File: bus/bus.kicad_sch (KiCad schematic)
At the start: 3 parts, among them J1 Conn_01x02, J2 Conn_01x15, J3 Conn_01x08

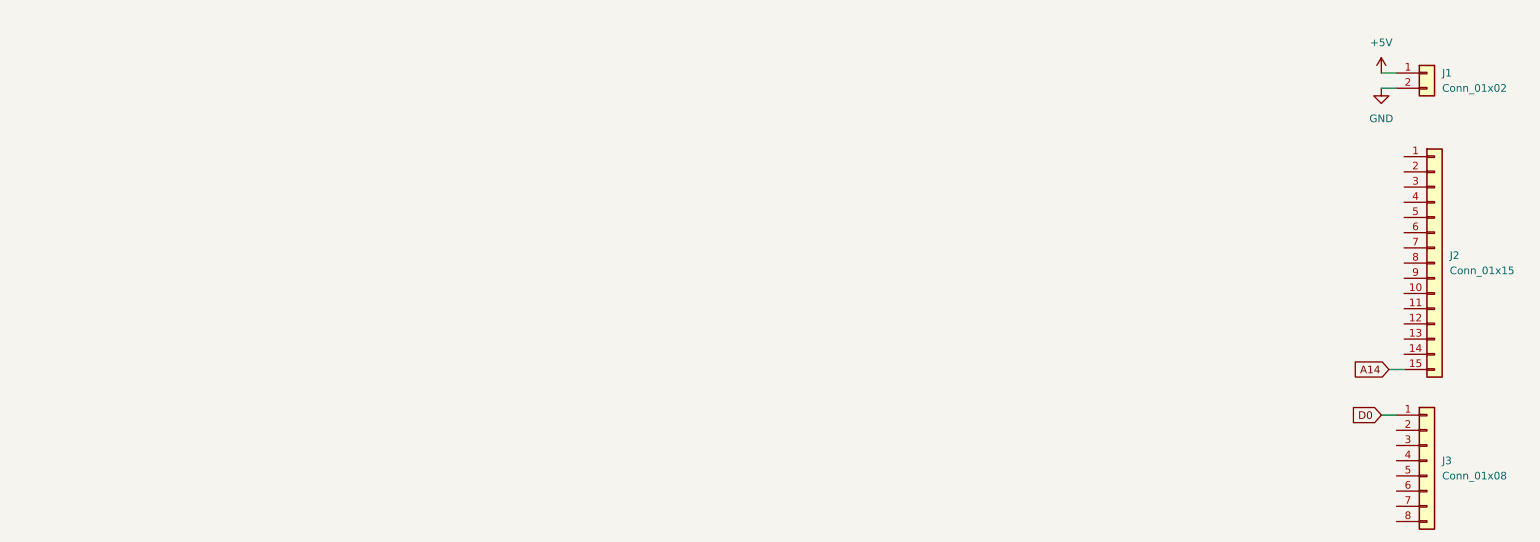
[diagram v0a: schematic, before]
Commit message: Done
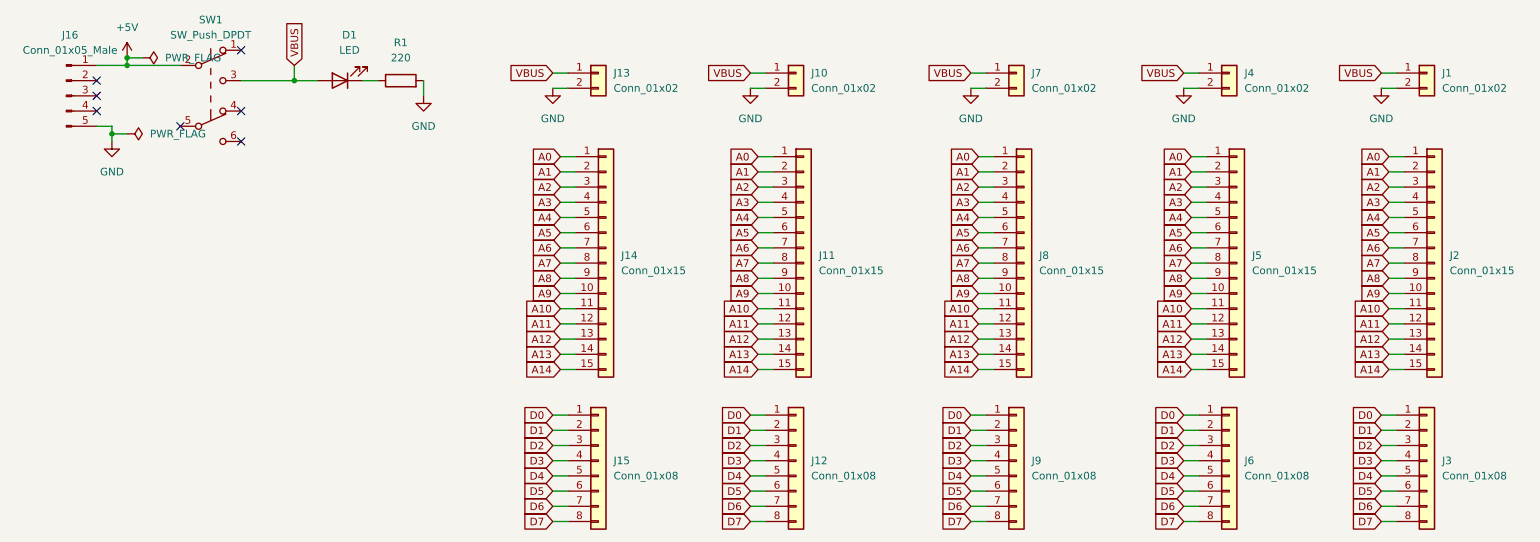
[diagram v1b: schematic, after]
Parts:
- added D1: LED, LED_THT:LED_D5.0mm, symbol Device:LED
- added J10, J13, J4, J7: Conn_01x02, Connector_PinSocket_2.54mm:PinSocket_1x02_P2.54mm_Vertical, symbol Connector_Generic:Conn_01x02
- added J11, J14, J5, J8: Conn_01x15, Connector_PinSocket_2.54mm:PinSocket_1x15_P2.54mm_Vertical, symbol Connector_Generic:Conn_01x15
- added J12, J15, J6, J9: Conn_01x08, Connector_PinSocket_2.54mm:PinSocket_1x08_P2.54mm_Vertical, symbol Connector_Generic:Conn_01x08
- added J16: Conn_01x05_Male, Connector_PinSocket_2.54mm:PinSocket_1x05_P2.54mm_Vertical, symbol Connector:Conn_01x05_Male
- added R1: 220, Resistor_THT:R_Axial_DIN0309_L9.0mm_D3.2mm_P12.70mm_Horizontal, symbol Device:R
- added SW1: SW_Push_DPDT, Button_Switch_THT:SW_E-Switch_EG1271_DPDT, symbol Switch:SW_Push_DPDT
- J1: footprint Connector_PinHeader_2.54mm:PinHeader_1x02_P2.54mm_Horizontal -> Connector_PinSocket_2.54mm:PinSocket_1x02_P2.54mm_Vertical
- J2: footprint Connector_PinHeader_2.54mm:PinHeader_1x15_P2.54mm_Horizontal -> Connector_PinSocket_2.54mm:PinSocket_1x15_P2.54mm_Vertical
- J3: footprint Connector_PinHeader_2.54mm:PinHeader_1x08_P2.54mm_Horizontal -> Connector_PinSocket_2.54mm:PinSocket_1x08_P2.54mm_Vertical
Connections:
- net +5V: now also J16.1 (Pin_1), SW1.2 (B); no longer J1.1 (Pin_1)
- net A14: now also J11.15 (Pin_15), J14.15 (Pin_15), J5.15 (Pin_15), J8.15 (Pin_15)
- net D0: now also J12.1 (Pin_1), J15.1 (Pin_1), J6.1 (Pin_1), J9.1 (Pin_1)
- net GND: now also J10.2 (Pin_2), J13.2 (Pin_2), J16.5 (Pin_5), J4.2 (Pin_2), J7.2 (Pin_2), R1.2
- net D1: now reaches J3.2 (Pin_2)
- net D1: now also J12.2 (Pin_2), J15.2 (Pin_2), J6.2 (Pin_2), J9.2 (Pin_2)
- net D2: now reaches J3.3 (Pin_3)
- net D2: now also J12.3 (Pin_3), J15.3 (Pin_3), J6.3 (Pin_3), J9.3 (Pin_3)
- net D3: now reaches J3.4 (Pin_4)
- net D3: now also J12.4 (Pin_4), J15.4 (Pin_4), J6.4 (Pin_4), J9.4 (Pin_4)
- net D4: now reaches J3.5 (Pin_5)
- net D4: now also J12.5 (Pin_5), J15.5 (Pin_5), J6.5 (Pin_5), J9.5 (Pin_5)
- net D5: now reaches J3.6 (Pin_6)
- net D5: now also J12.6 (Pin_6), J15.6 (Pin_6), J6.6 (Pin_6), J9.6 (Pin_6)
- net D6: now reaches J3.7 (Pin_7)
- net D6: now also J12.7 (Pin_7), J15.7 (Pin_7), J6.7 (Pin_7), J9.7 (Pin_7)
- net D7: now reaches J3.8 (Pin_8)
- net D7: now also J12.8 (Pin_8), J15.8 (Pin_8), J6.8 (Pin_8), J9.8 (Pin_8)
- net A0: now reaches J2.1 (Pin_1)
- net A0: now also J11.1 (Pin_1), J14.1 (Pin_1), J5.1 (Pin_1), J8.1 (Pin_1)
- net A9: now reaches J2.10 (Pin_10)
- net A9: now also J11.10 (Pin_10), J14.10 (Pin_10), J5.10 (Pin_10), J8.10 (Pin_10)
- net A10: now reaches J2.11 (Pin_11)
- net A10: now also J11.11 (Pin_11), J14.11 (Pin_11), J5.11 (Pin_11), J8.11 (Pin_11)
- net A11: now reaches J2.12 (Pin_12)
- net A11: now also J11.12 (Pin_12), J14.12 (Pin_12), J5.12 (Pin_12), J8.12 (Pin_12)
- net A12: now reaches J2.13 (Pin_13)
- net A12: now also J11.13 (Pin_13), J14.13 (Pin_13), J5.13 (Pin_13), J8.13 (Pin_13)
- net A13: now reaches J2.14 (Pin_14)
- net A13: now also J11.14 (Pin_14), J14.14 (Pin_14), J5.14 (Pin_14), J8.14 (Pin_14)
- net A1: now reaches J2.2 (Pin_2)
- net A1: now also J11.2 (Pin_2), J14.2 (Pin_2), J5.2 (Pin_2), J8.2 (Pin_2)
- net A2: now reaches J2.3 (Pin_3)
- net A2: now also J11.3 (Pin_3), J14.3 (Pin_3), J5.3 (Pin_3), J8.3 (Pin_3)
- net A3: now reaches J2.4 (Pin_4)
- net A3: now also J11.4 (Pin_4), J14.4 (Pin_4), J5.4 (Pin_4), J8.4 (Pin_4)
- net A4: now reaches J2.5 (Pin_5)
- net A4: now also J11.5 (Pin_5), J14.5 (Pin_5), J5.5 (Pin_5), J8.5 (Pin_5)
- net A5: now reaches J2.6 (Pin_6)
- net A5: now also J11.6 (Pin_6), J14.6 (Pin_6), J5.6 (Pin_6), J8.6 (Pin_6)
- net A6: now reaches J2.7 (Pin_7)
- net A6: now also J11.7 (Pin_7), J14.7 (Pin_7), J5.7 (Pin_7), J8.7 (Pin_7)
- net A7: now reaches J2.8 (Pin_8)
- net A7: now also J11.8 (Pin_8), J14.8 (Pin_8), J5.8 (Pin_8), J8.8 (Pin_8)
- net A8: now reaches J2.9 (Pin_9)
- net A8: now also J11.9 (Pin_9), J14.9 (Pin_9), J5.9 (Pin_9), J8.9 (Pin_9)
- new net: D1.1 (K), R1.1
- new net VBUS: D1.2 (A), J1.1 (Pin_1), J10.1 (Pin_1), J13.1 (Pin_1), J4.1 (Pin_1), J7.1 (Pin_1), SW1.3 (C)
- no-connect marks 0 -> 7
